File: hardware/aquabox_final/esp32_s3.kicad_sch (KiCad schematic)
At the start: 1 part, among them U2 ESP32-S3-DEVKITC-1-N16R8V

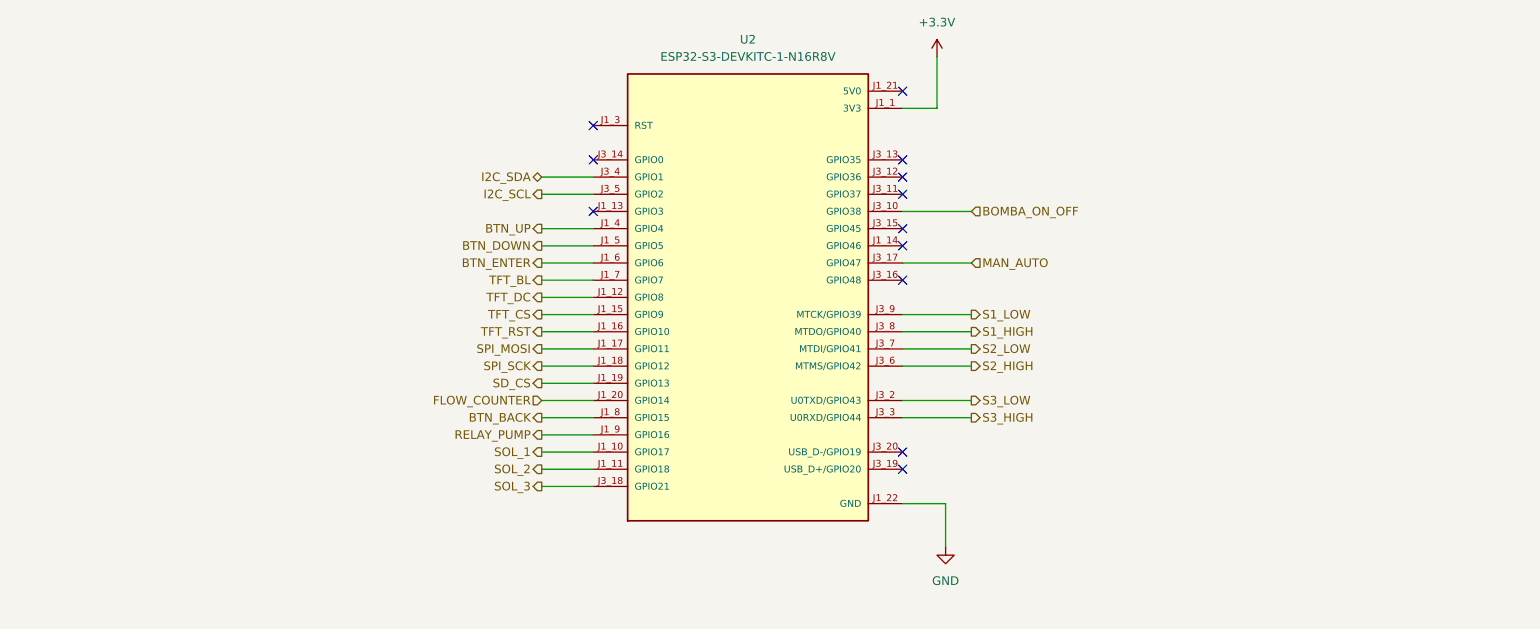
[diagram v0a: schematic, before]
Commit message: Atualização
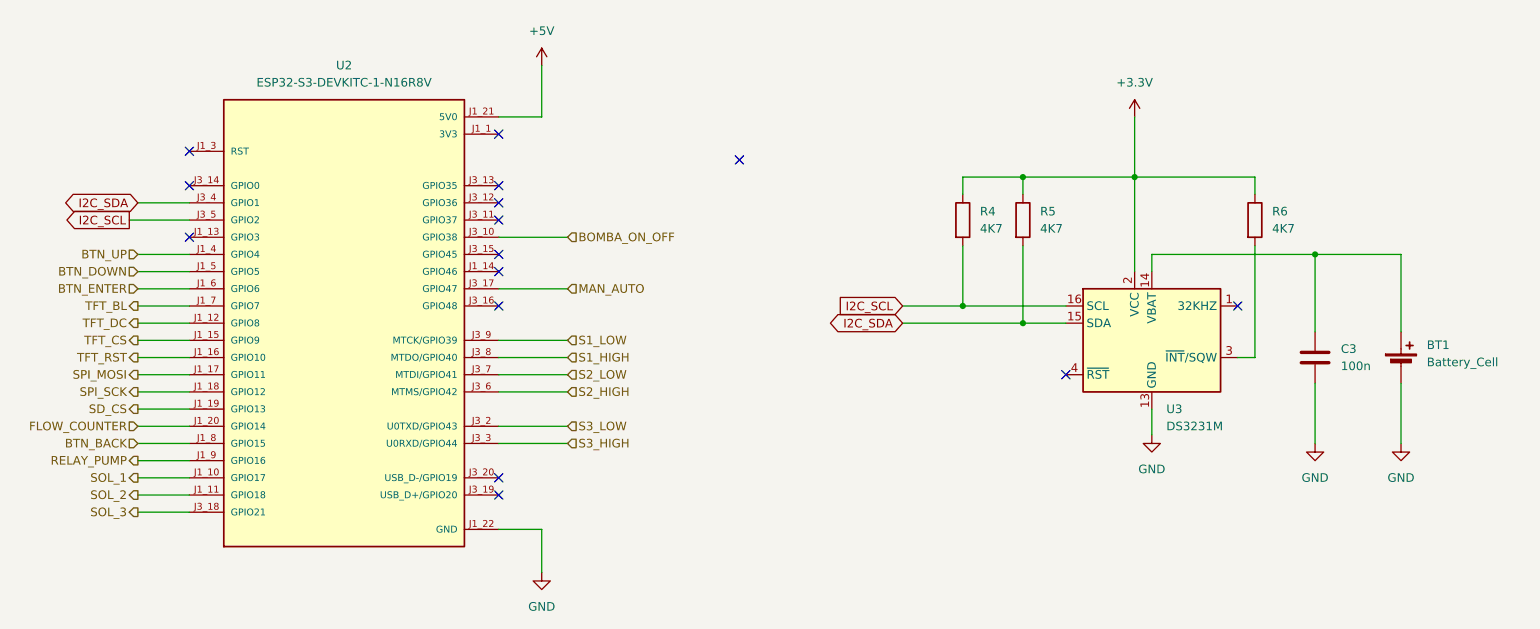
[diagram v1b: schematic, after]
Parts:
- added BT1: Battery_Cell, Battery:Battery_Panasonic_CR2032-HFN_Horizontal_CircularHoles, symbol Device:Battery_Cell
- added C3: 100n, symbol Device:C
- added R4, R5, R6: 4K7, symbol Device:R
- added U3: DS3231M, Package_SO:SOIC-16W_7.5x10.3mm_P1.27mm, symbol Timer_RTC:DS3231M
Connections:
- net +3.3V: now also R4.1, R5.1, R6.1, U3.2 (VCC); no longer U2.J1_1 (3V3), U2.J1_2 (3V3)
- net GND: now also BT1.2 (-), C3.2, U3.10 (GND), U3.11 (GND), U3.12 (GND), U3.13 (GND), U3.5 (GND), U3.6 (GND), U3.7 (GND), U3.8 (GND), U3.9 (GND)
- net I2C_SCL: now also R4.2, U3.16 (SCL)
- net I2C_SDA: now also R5.2, U3.15 (SDA)
- net +5V: now reaches U2.J1_21 (5V0)
- new net: BT1.1 (+), C3.1, U3.14 (VBAT)
- new net: R6.2, U3.3 (~{INT}/SQW)
- new net 3V3: U2.J1_1 (3V3), U2.J1_2 (3V3)
- no-connect marks 12 -> 15
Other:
- moved on the sheet: U2
